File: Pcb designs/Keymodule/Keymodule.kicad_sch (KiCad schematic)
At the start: 105 parts, among them J1 USB connect, U1 RP2040, U2 SN74LV1T34DBV, U3 AMS1117-3.3, U4 W25Q128JVS, Y1 ABM8-272-T3

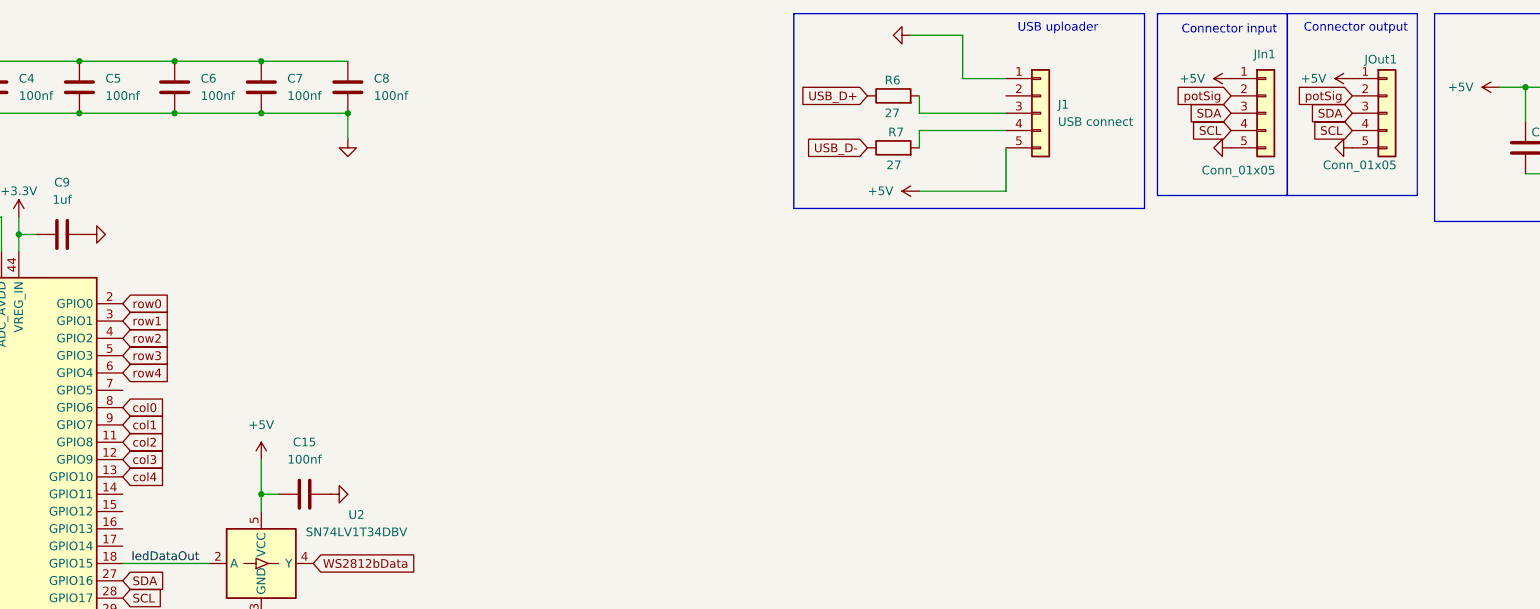
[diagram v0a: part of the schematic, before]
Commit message: Almost done
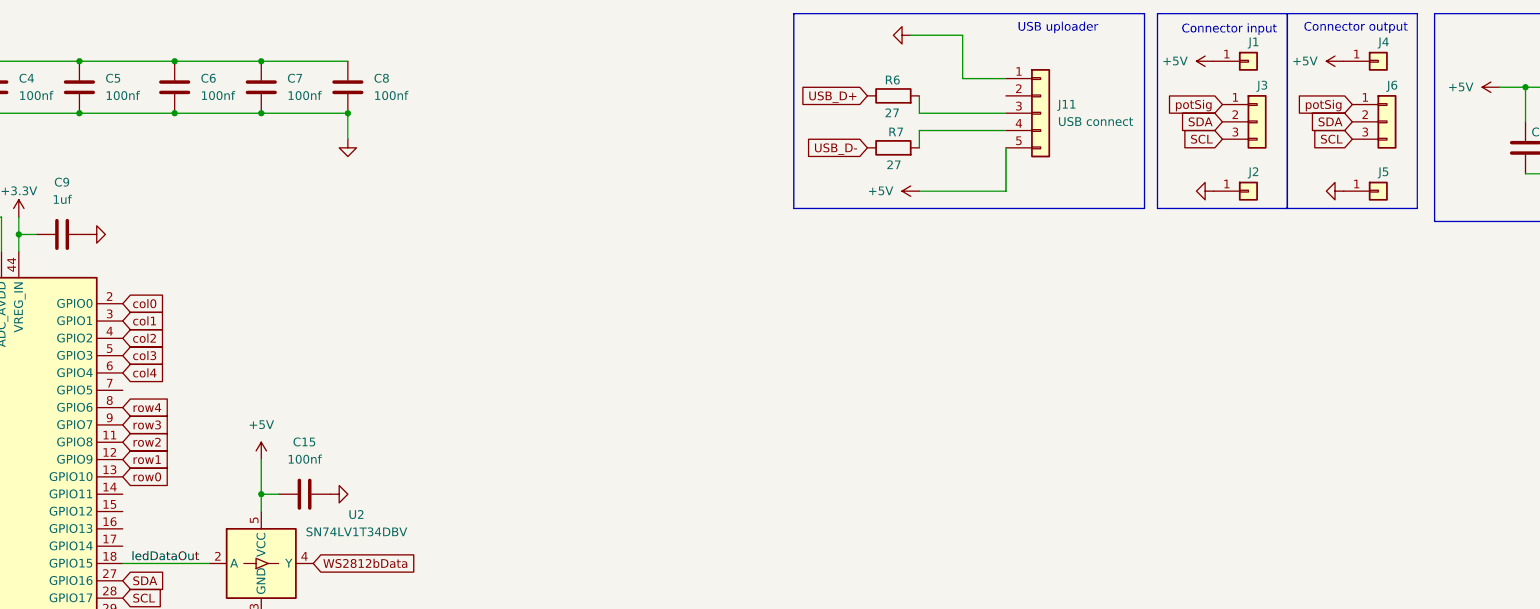
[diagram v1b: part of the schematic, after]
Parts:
- removed JIn1: Conn_01x05, Connector_PinSocket_2.00mm:PinSocket_1x05_P2.00mm_Horizontal, symbol Connector_Generic:Conn_01x05
- removed JOut1: Conn_01x05, 1_Custom_library:Magnetic pogo out, symbol Connector_Generic:Conn_01x05
- added J1, J2, J4, J5: Conn_01x01, Connector_PinHeader_1.27mm:PinHeader_1x01_P1.27mm_Horizontal, symbol Connector_Generic:Conn_01x01
- added J3, J6: Conn_01x03, Connector_PinHeader_1.27mm:PinHeader_1x03_P1.27mm_Horizontal, symbol Connector_Generic:Conn_01x03
- renumbered J1 to J11
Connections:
- net +5V: now also J1.1 (Pin_1), J4.1 (Pin_1)
- net GND: now also J2.1 (Pin_1), J5.1 (Pin_1)
- net SCL: now also J3.3 (Pin_3), J6.3 (Pin_3)
- net SDA: now also J3.2 (Pin_2), J6.2 (Pin_2)
- net col0: now also U1.2 (GPIO0); no longer U1.8 (GPIO6)
- net col1: now also U1.3 (GPIO1); no longer U1.9 (GPIO7)
- net col2: now also U1.4 (GPIO2); no longer U1.11 (GPIO8)
- net col3: now also U1.5 (GPIO3); no longer U1.12 (GPIO9)
- net col4: now also U1.6 (GPIO4); no longer U1.13 (GPIO10)
- net potSig: now also J3.1 (Pin_1), J6.1 (Pin_1)
- net row0: now also U1.13 (GPIO10); no longer U1.2 (GPIO0)
- net row1: now also U1.12 (GPIO9); no longer U1.3 (GPIO1)
- net row2: now also U1.11 (GPIO8); no longer U1.4 (GPIO2)
- net row3: now also U1.9 (GPIO7); no longer U1.5 (GPIO3)
- net row4: now also U1.8 (GPIO6); no longer U1.6 (GPIO4)
